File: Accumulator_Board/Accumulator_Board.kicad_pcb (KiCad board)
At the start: 2 copper layers, 125.7 x 89.5 mm, 98 parts, among them J1 IMD, J10 HVIL, J11 Molex Nanofit 16pin, J2 Molex Nanofit 12pin, J4 Current Sensor, J5 IsoSPI, J6 Shutdown IL, J7 AIRs Power, J8 Precharge Resistor, J9 TS+/TS-, K1 DK1A1B-12V, K2 G5PZ-1A-X DC12, K3 DK1A1B-12V, K4 G6BK-1114P-US, Q1 STS6NF20V, Q2 STS6NF20V, U1 ISO1050DUB, U10 MC7809CTG, U12 LM555xN, U15 ZXTR2005ZQ-13, U16 4069, U2 NUCLEO-L432KC, U3 4069, U4 SN74HCS32DR, U5 MCP6004, U6 DS18B20U, U7 HEF4093B, U8 LTC6820, U9 L7805CV

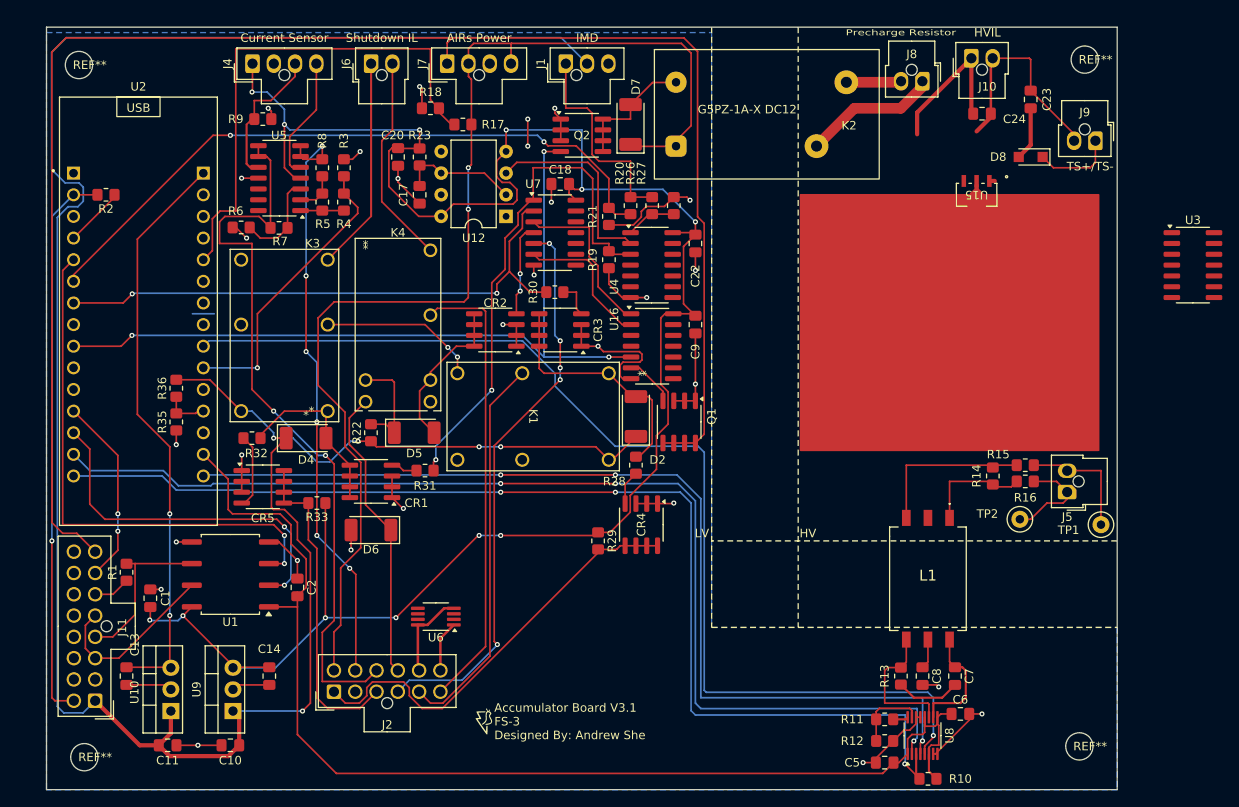
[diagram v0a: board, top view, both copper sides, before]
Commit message: Accumulator_Board-V4
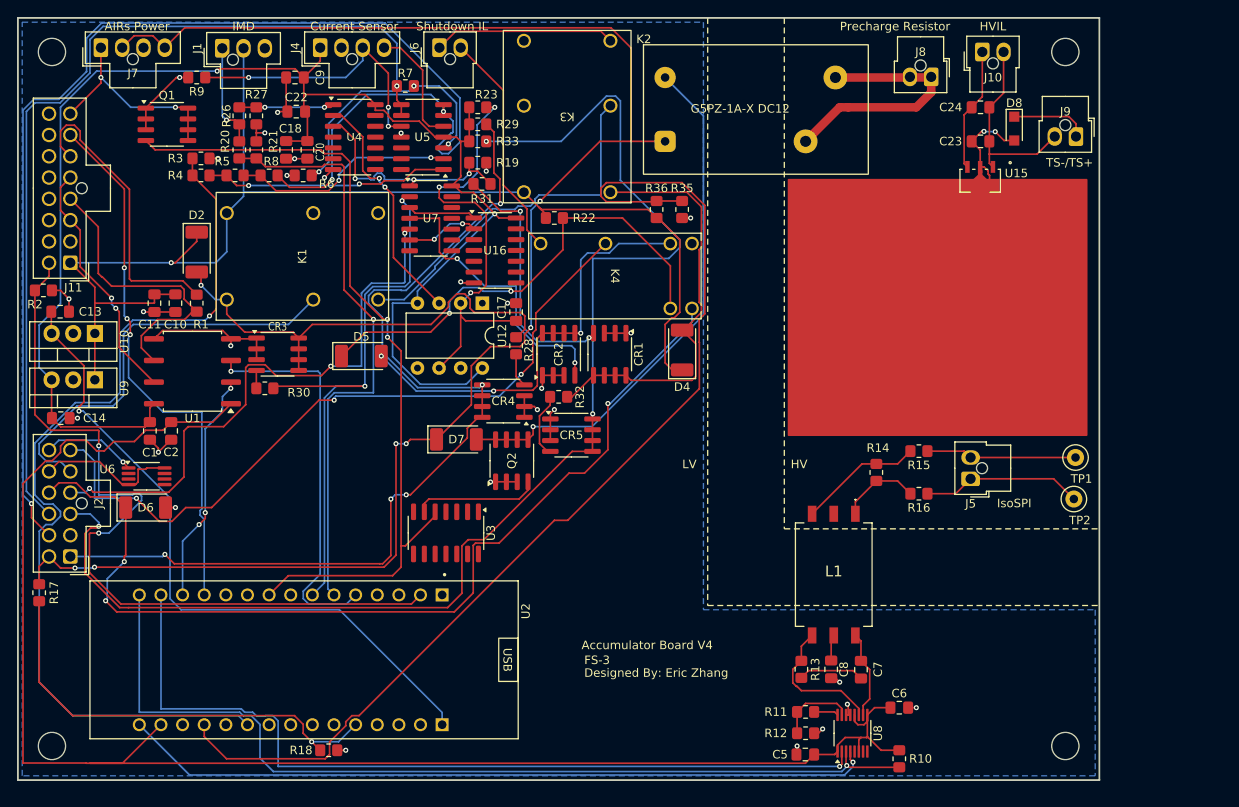
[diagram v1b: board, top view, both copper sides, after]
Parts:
- removed G***: LOGO, FS_3_Global_Footprint_Library:FORMULA SLUG
- removed the REF** at (27.3, 107.3)
- removed the REF** at (144.1, 106.0)
- removed the REF** at (144.8, 25.4)
- removed the REF** at (26.7, 26.0)
- added REF**: MountingHole_3.2mm_M3, MountingHole:MountingHole_3.2mm_M3, F.Cu at (142.5, 24.5)
- added REF**: MountingHole_3.2mm_M3, MountingHole:MountingHole_3.2mm_M3, F.Cu at (142.5, 106.0)
- added REF**: MountingHole_3.2mm_M3, MountingHole:MountingHole_3.2mm_M3, F.Cu at (23.5, 106.0)
- added REF**: MountingHole_3.2mm_M3, MountingHole:MountingHole_3.2mm_M3, F.Cu at (23.5, 24.5)
- J9: value TS+/TS- -> TS-/TS+
- moved U3 93.2 mm to (69.8, 81.0), turned to -90 degrees
- moved R18 76.3 mm to (56.0, 106.5), turned to 0 degrees
- moved R17 74.2 mm to (22.0, 88.0), turned to -90 degrees
- moved Q1 69.6 mm to (37.0, 33.0), turned to 0 degrees
- moved R35 64.4 mm to (97.5, 43.0)
- moved R36 60.2 mm to (94.5, 43.0), turned to -90 degrees
- moved C9 55.3 mm to (52.0, 27.5), turned to 0 degrees
- moved D2 55.1 mm to (40.5, 48.0), turned to -90 degrees
- moved C10 52.3 mm to (38.0, 54.0), turned to -90 degrees
- moved C11 51.9 mm to (35.5, 54.0), turned to -90 degrees
- moved J11 51.5 mm to (25.7, 49.2)
- moved R29 50.9 mm to (73.5, 33.0), turned to 0 degrees
- moved R27 50.1 mm to (47.5, 32.0), turned to -90 degrees
- moved R26 49.6 mm to (45.5, 32.0), turned to 90 degrees
- moved C22 49.4 mm to (52.2, 31.5), turned to 0 degrees
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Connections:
- J8 pad 1: Net-(J8-Pad1) -> Net-(J8-Pad2)
- K2 pad 2: Net-(J8-Pad1) -> Net-(J8-Pad2)
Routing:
- net /IR+_GND: track 192.7 -> 24.8 mm, vias 0 -> 2
- net +12V: track 285.8 -> 147.5 mm, vias 5 -> 1
- net /BMS_CS: track 127.6 -> 0.00 mm, vias 1 -> 0
- net /GLV Voltage: track 4.60 -> 125.9 mm
- net /IMD_LED_Control: track 38.3 -> 154.8 mm, vias 0 -> 3
- net /Current_Vref: track 70.2 -> 157.3 mm, vias 6 -> 3
- net /SH_RESET: track 34.7 -> 114.1 mm, vias 0 -> 3
- net /Amp_Curr_Sensor: track 34.4 -> 108.7 mm
- net /BMS_LED_Control: track 49.8 -> 115.3 mm, vias 0 -> 5
- net GND: track 146.4 -> 84.4 mm
- net +5V: track 235.8 -> 175.0 mm, vias 12 -> 2
- net /IR+_12V: track 138.6 -> 190.2 mm, vias 2 -> 6
- net +3.3V: track 138.9 -> 188.2 mm
- net Net-(D7-A): track 14.5 -> 63.1 mm, vias 0 -> 1
- net Net-(D5-K): track 12.6 -> 56.0 mm, vias 0 -> 2
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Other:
- board size 125.7 x 89.5 mm -> 127 x 89.5 mm
- board text added: "Accumulator Board V4"
- board text added: "Designed By: Eric Zhang"
- board text added: "FS-3"
- board text removed: "Accumulator Board V3.1 FS-3 Designed By: Andrew She"
